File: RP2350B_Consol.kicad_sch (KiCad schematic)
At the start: 33 parts, among them J1 Conn_01x15_Socket, J10 VGA, J2 Conn_01x15_Socket, J3 Conn_01x15_Socket, J4 Conn_01x15_Socket, J5 Conn_02x06_Odd_Even, J6 Conn_02x20_Odd_Even, J7 NES_Joystick1, J8 NES_Joystick2, J9 PJ320D, U2 SN76489AN

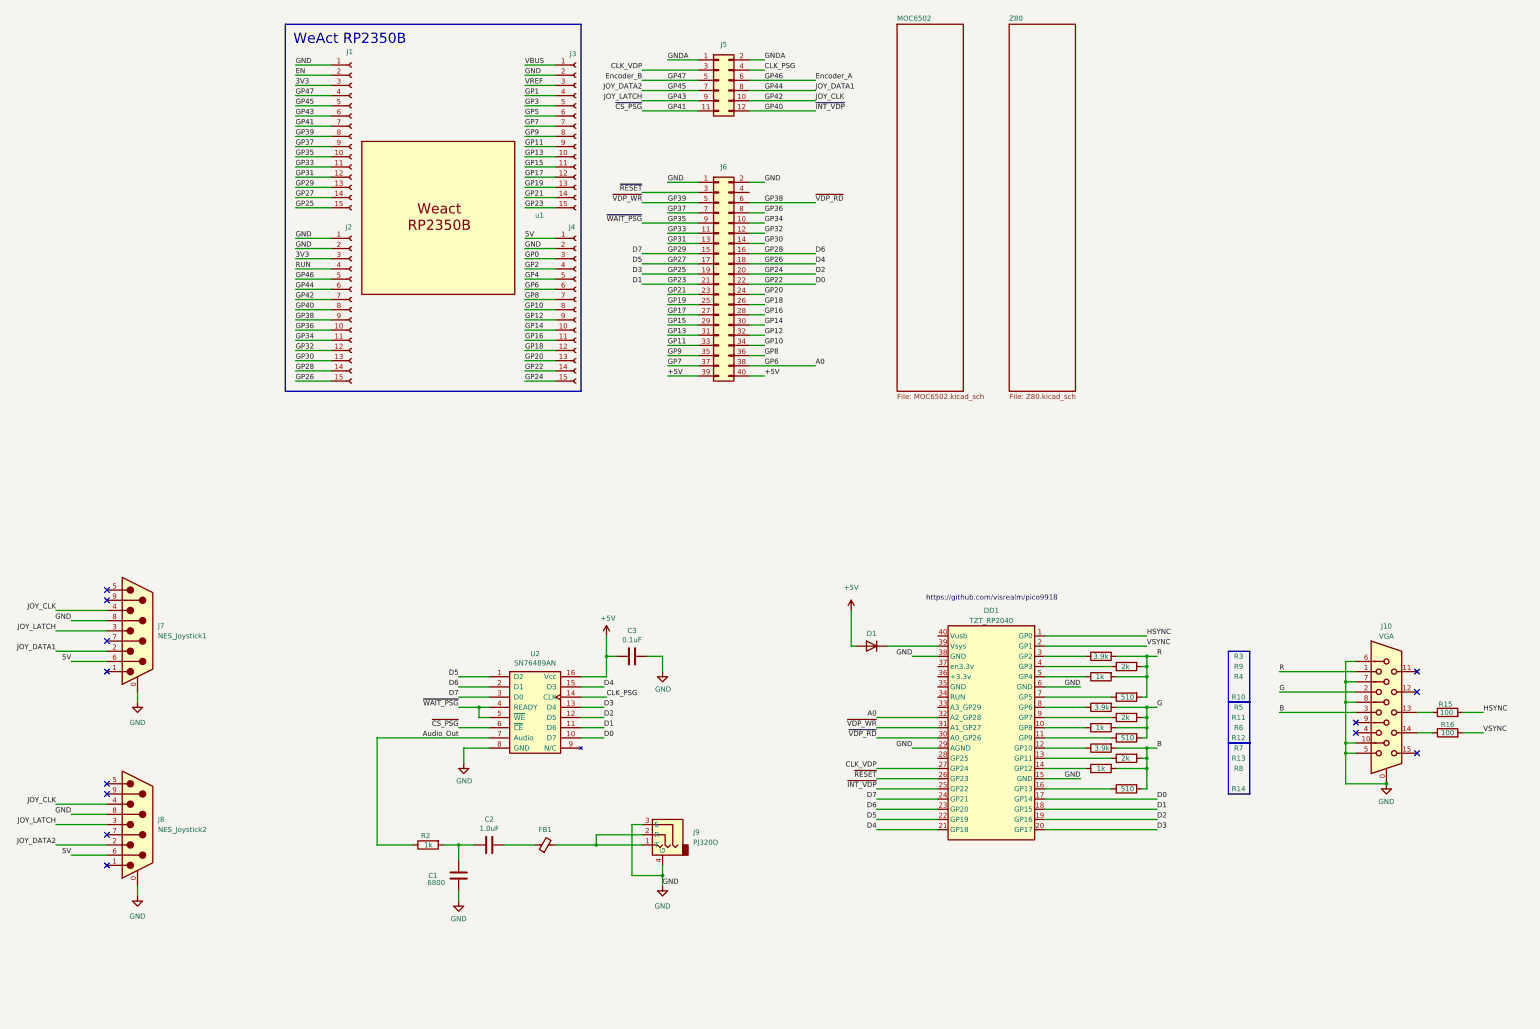
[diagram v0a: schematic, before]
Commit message: Update RP2350B_Consol.kicad_sch
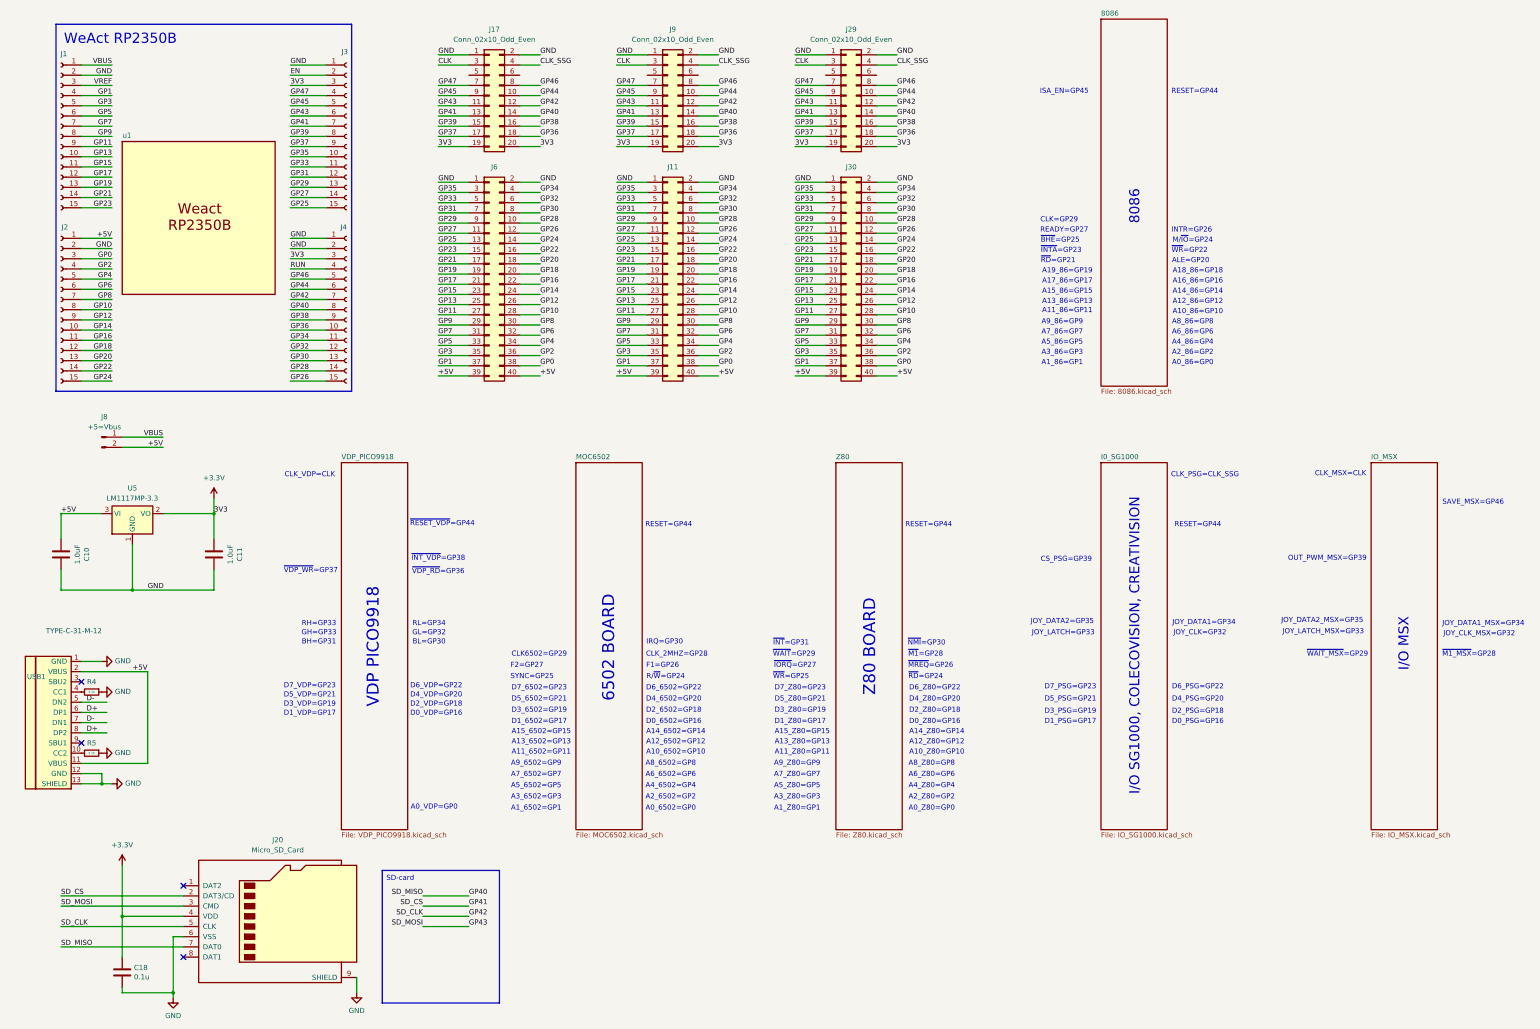
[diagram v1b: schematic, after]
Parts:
- removed C1: 6800, Capacitor_SMD:C_0805_2012Metric_Pad1.18x1.45mm_HandSolder, symbol Device:C
- removed C2: 1.0uF, Capacitor_SMD:C_0805_2012Metric_Pad1.18x1.45mm_HandSolder, symbol Device:C
- removed C3: 0.1uF, Capacitor_SMD:C_0805_2012Metric_Pad1.18x1.45mm_HandSolder, symbol Device:C
- removed D1: D, Diode_SMD:D_1206_3216Metric_Pad1.42x1.75mm_HandSolder, symbol Device:D
- removed DD1: TZT_RP2040, Library:RP2040_purple_allPin, symbol Watapico:GreatztRP2040_Purple
- removed FB1: FerriteBead_Small, Inductor_SMD:L_0805_2012Metric_Pad1.15x1.40mm_HandSolder, symbol Device:FerriteBead_Small
- removed J10: VGA, Connector_Dsub:DSUB-15-HD_Female_Horizontal_P2.29x1.98mm_EdgePinOffset3.03mm_Housed_MountingHolesOffset4.94mm, symbol Connector:DB15_Female_HighDensity_MountingHoles
- removed J5: Conn_02x06_Odd_Even, UM6502:EDGE_2x12, symbol Connector_Generic:Conn_02x06_Odd_Even
- removed J7: NES_Joystick1, Connector_Dsub:DSUB-9_Male_Vertical_P2.77x2.84mm_MountingHoles, symbol Connector:DE9_Plug_MountingHoles
- removed J8: NES_Joystick2, Connector_Dsub:DSUB-9_Male_Vertical_P2.77x2.84mm_MountingHoles, symbol Connector:DE9_Plug_MountingHoles
- removed J9: PJ320D, Library:PJ320D_3.5mm_Jack, symbol Connector_Audio:AudioJack3_Ground
- removed R10, R12, R14: 510, Resistor_SMD:R_0805_2012Metric_Pad1.20x1.40mm_HandSolder, symbol Device:R
- removed R11, R13, R9: 2k, Resistor_SMD:R_0805_2012Metric_Pad1.20x1.40mm_HandSolder, symbol Device:R
- removed R15, R16: 100, Resistor_SMD:R_0805_2012Metric_Pad1.20x1.40mm_HandSolder, symbol Device:R
- removed R2, R4, R6, R8: 1k, Resistor_SMD:R_0805_2012Metric_Pad1.20x1.40mm_HandSolder, symbol Device:R
- removed R3, R5, R7: 3.9k, Resistor_SMD:R_0805_2012Metric_Pad1.20x1.40mm_HandSolder, symbol Device:R
- removed U2: SN76489AN, Package_DIP:DIP-16_W7.62mm_LongPads, symbol LeakoChips:SN76489AN
- added C10, C11: 1.0uF, Capacitor_SMD:C_0805_2012Metric_Pad1.18x1.45mm_HandSolder, symbol Device:C
- added C18: 0.1u, Capacitor_SMD:C_0805_2012Metric_Pad1.18x1.45mm_HandSolder, symbol Device:C
- added J11, J30: Conn_02x20_Odd_Even, Connector_PinSocket_2.54mm:PinSocket_2x20_P2.54mm_Vertical, symbol Connector_Generic:Conn_02x20_Odd_Even
- added J17, J29, J9: Conn_02x10_Odd_Even, Connector_PinSocket_2.54mm:PinSocket_2x10_P2.54mm_Vertical, symbol Connector_Generic:Conn_02x10_Odd_Even
- added J20: Micro_SD_Card, Library:GCT-MEM2055-00-190-01-A, symbol Connector:Micro_SD_Card
- added J8: +5=Vbus, Connector_PinHeader_2.54mm:PinHeader_1x02_P2.54mm_Vertical, symbol Connector:Conn_01x02_Pin
- added R4, R5: 5.1K, Resistor_SMD:R_0805_2012Metric_Pad1.20x1.40mm_HandSolder, symbol Device:R_Small
- added U5: LM1117MP-3.3, Package_TO_SOT_SMD:SOT-223-3_TabPin2, symbol Regulator_Linear:LM1117MP-3.3
- added USB1: TYPE-C-31-M-12, Library:USB-TYPE-C-31-M-12_lib2, symbol Type-C:HRO-TYPE-C-31-M-12
- J6: footprint UM6502:EDGE_2x20 -> Connector_PinSocket_2.54mm:PinSocket_2x20_P2.54mm_Vertical
- u1: footprint RP2350B_WeAct:RP2350B_WeAct -> Library:RP2350B_WeAct
- renumbered J3 to J1, J4 to J2, J1 to J3, J2 to J4
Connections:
- net 5V is gone; now on net +5V: J2.1 (Pin_1)
- net ~{RESET} is gone; now on net GP35: J6.3 (Pin_3)
- net +5V: now also C10.2, J11.39 (Pin_39), J11.40 (Pin_40), J30.39 (Pin_39), J30.40 (Pin_40), J8.2 (Pin_2), U5.3 (VI), USB1.11 (VBUS), USB1.2 (VBUS)
- net GND: now also C10.1, C11.1, C18.2, J11.1 (Pin_1), J11.2 (Pin_2), J17.1 (Pin_1), J17.2 (Pin_2), J20.6 (VSS), J20.9 (SHIELD), J29.1 (Pin_1), J29.2 (Pin_2), J30.1 (Pin_1), J30.2 (Pin_2), J9.1 (Pin_1), J9.2 (Pin_2), R4.1, R5.1, U5.1 (GND), USB1.1 (GND), USB1.12 (GND), USB1.13 (SHIELD)
- net GP0: now also J6.38 (Pin_38), J11.38 (Pin_38), J30.38 (Pin_38)
- net GP1: now also J6.37 (Pin_37), J11.37 (Pin_37), J30.37 (Pin_37)
- net GP10: now also J6.28 (Pin_28), J11.28 (Pin_28), J30.28 (Pin_28); no longer J6.34 (Pin_34)
- net GP11: now also J6.27 (Pin_27), J11.27 (Pin_27), J30.27 (Pin_27); no longer J6.33 (Pin_33)
- net GP12: now also J6.26 (Pin_26), J11.26 (Pin_26), J30.26 (Pin_26); no longer J6.32 (Pin_32)
- net GP13: now also J6.25 (Pin_25), J11.25 (Pin_25), J30.25 (Pin_25); no longer J6.31 (Pin_31)
- net GP14: now also J6.24 (Pin_24), J11.24 (Pin_24), J30.24 (Pin_24); no longer J6.30 (Pin_30)
- net GP15: now also J6.23 (Pin_23), J11.23 (Pin_23), J30.23 (Pin_23); no longer J6.29 (Pin_29)
- net GP16: now also J6.22 (Pin_22), J11.22 (Pin_22), J30.22 (Pin_22); no longer J6.28 (Pin_28)
- net GP17: now also J6.21 (Pin_21), J11.21 (Pin_21), J30.21 (Pin_21); no longer J6.27 (Pin_27)
- net GP18: now also J6.20 (Pin_20), J11.20 (Pin_20), J30.20 (Pin_20); no longer J6.26 (Pin_26)
- net GP19: now also J6.19 (Pin_19), J11.19 (Pin_19), J30.19 (Pin_19); no longer J6.25 (Pin_25)
- net GP2: now also J6.36 (Pin_36), J11.36 (Pin_36), J30.36 (Pin_36)
- net GP20: now also J6.18 (Pin_18), J11.18 (Pin_18), J30.18 (Pin_18); no longer J6.24 (Pin_24)
- net GP21: now also J6.17 (Pin_17), J11.17 (Pin_17), J30.17 (Pin_17); no longer J6.23 (Pin_23)
- net GP3: now also J6.35 (Pin_35), J11.35 (Pin_35), J30.35 (Pin_35)
- net GP30: now also J6.8 (Pin_8), J11.8 (Pin_8), J30.8 (Pin_8); no longer J6.14 (Pin_14)
- net GP31: now also J6.7 (Pin_7), J11.7 (Pin_7), J30.7 (Pin_7); no longer J6.13 (Pin_13)
- net GP32: now also J6.6 (Pin_6), J11.6 (Pin_6), J30.6 (Pin_6); no longer J6.12 (Pin_12)
- net GP33: now also J6.5 (Pin_5), J11.5 (Pin_5), J30.5 (Pin_5); no longer J6.11 (Pin_11)
- net GP34: now also J6.4 (Pin_4), J11.4 (Pin_4), J30.4 (Pin_4); no longer J6.10 (Pin_10)
- net GP35: now also J11.3 (Pin_3), J30.3 (Pin_3); no longer J6.9 (Pin_9)
- net GP36: now also J17.18 (Pin_18), J29.18 (Pin_18), J9.18 (Pin_18); no longer J6.8 (Pin_8)
- net GP37: now also J17.17 (Pin_17), J29.17 (Pin_17), J9.17 (Pin_17); no longer J6.7 (Pin_7)
- net GP38: now also J17.16 (Pin_16), J29.16 (Pin_16), J9.16 (Pin_16); no longer J6.6 (Pin_6)
- net GP39: now also J17.15 (Pin_15), J29.15 (Pin_15), J9.15 (Pin_15); no longer J6.5 (Pin_5)
- net GP4: now also J6.34 (Pin_34), J11.34 (Pin_34), J30.34 (Pin_34)
- net GP40: now also J17.14 (Pin_14), J20.7 (DAT0), J29.14 (Pin_14), J9.14 (Pin_14)
- net GP41: now also J17.13 (Pin_13), J20.2 (DAT3/CD), J29.13 (Pin_13), J9.13 (Pin_13)
- net GP42: now also J17.12 (Pin_12), J20.5 (CLK), J29.12 (Pin_12), J9.12 (Pin_12)
- net GP43: now also J17.11 (Pin_11), J20.3 (CMD), J29.11 (Pin_11), J9.11 (Pin_11)
- net GP44: now also J17.10 (Pin_10), J29.10 (Pin_10), J9.10 (Pin_10)
- net GP45: now also J17.9 (Pin_9), J29.9 (Pin_9), J9.9 (Pin_9)
- net GP5: now also J6.33 (Pin_33), J11.33 (Pin_33), J30.33 (Pin_33)
- net GP7: now also J6.31 (Pin_31), J11.31 (Pin_31), J30.31 (Pin_31); no longer J6.37 (Pin_37)
- net GP8: now also J6.30 (Pin_30), J11.30 (Pin_30), J30.30 (Pin_30); no longer J6.36 (Pin_36)
- net GP9: now also J6.29 (Pin_29), J11.29 (Pin_29), J30.29 (Pin_29); no longer J6.35 (Pin_35)
- net VBUS: now also J8.1 (Pin_1)
- net 3V3 renamed +3.3V
- net +3.3V: now also C11.2, C18.1, J17.19 (Pin_19), J17.20 (Pin_20), J20.4 (VDD), J29.19 (Pin_19), J29.20 (Pin_20), J9.19 (Pin_19), J9.20 (Pin_20), U5.2 (VO)
- net A0 renamed GP6
- net GP6: now also J6.32 (Pin_32), J11.32 (Pin_32), J30.32 (Pin_32); no longer J6.38 (Pin_38)
- net D0 renamed GP22
- net GP22: now also J6.16 (Pin_16), J11.16 (Pin_16), J30.16 (Pin_16); no longer J6.22 (Pin_22)
- net D1 renamed GP23
- net GP23: now also J6.15 (Pin_15), J11.15 (Pin_15), J30.15 (Pin_15); no longer J6.21 (Pin_21)
- net D2 renamed GP24
- net GP24: now also J6.14 (Pin_14), J11.14 (Pin_14), J30.14 (Pin_14); no longer J6.20 (Pin_20)
- net D3 renamed GP25
- net GP25: now also J6.13 (Pin_13), J11.13 (Pin_13), J30.13 (Pin_13); no longer J6.19 (Pin_19)
- net D4 renamed GP26
- net GP26: now also J6.12 (Pin_12), J11.12 (Pin_12), J30.12 (Pin_12); no longer J6.18 (Pin_18)
- net D5 renamed GP27
- net GP27: now also J6.11 (Pin_11), J11.11 (Pin_11), J30.11 (Pin_11); no longer J6.17 (Pin_17)
- net D6 renamed GP28
- net GP28: now also J6.10 (Pin_10), J11.10 (Pin_10), J30.10 (Pin_10); no longer J6.16 (Pin_16)
- net D7 renamed GP29
- net GP29: now also J6.9 (Pin_9), J11.9 (Pin_9), J30.9 (Pin_9); no longer J6.15 (Pin_15)
- net Encoder_A renamed GP46
- net GP46: now also J17.8 (Pin_8), J29.8 (Pin_8), J9.8 (Pin_8)
- net Encoder_B renamed GP47
- net GP47: now also J17.7 (Pin_7), J29.7 (Pin_7), J9.7 (Pin_7)
- new net: R4.2, USB1.4 (CC1)
- new net: R5.2, USB1.10 (CC2)
- new net CLK: J17.3 (Pin_3), J29.3 (Pin_3), J9.3 (Pin_3)
- new net CLK_SSG: J17.4 (Pin_4), J29.4 (Pin_4), J9.4 (Pin_4)
- new net D+: USB1.6 (DP1), USB1.8 (DP2)
- new net D-: USB1.5 (DN2), USB1.7 (DN1)
- no-connect marks 13 -> 4
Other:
- added sheet 8086 (8086.kicad_sch)
- added sheet I0_SG1000 (IO_SG1000.kicad_sch)
- added sheet IO_MSX (IO_MSX.kicad_sch)
- added sheet VDP_PICO9918 (VDP_PICO9918.kicad_sch)
- note added: "6502 BOARD"
- note added: "8086"
- note added: "A0_6502=GP0"
- note added: "A0_86=GP0"
- note added: "A0_VDP=GP0"
- note added: "A0_Z80=GP0"
- note added: "A10_6502=GP10"
- note added: "A10_86=GP10"
- note added: "A10_Z80=GP10"
- note added: "A11_6502=GP11"
- note added: "A11_86=GP11"
- note added: "A11_Z80=GP11"
- note added: "A12_6502=GP12"
- note added: "A12_86=GP12"
- note added: "A12_Z80=GP12"
- note added: "A13_6502=GP13"
- note added: "A13_86=GP13"
- note added: "A13_Z80=GP13"
- note added: "A14_6502=GP14"
- note added: "A14_86=GP14"
- note added: "A14_Z80=GP14"
- note added: "A15_6502=GP15"
- note added: "A15_86=GP15"
- note added: "A15_Z80=GP15"
- note added: "A16_86=GP16"
- note added: "A17_86=GP17"
- note added: "A18_86=GP18"
- note added: "A19_86=GP19"
- note added: "A1_6502=GP1"
- note added: "A1_86=GP1"
- note added: "A1_Z80=GP1"
- note added: "A2_6502=GP2"
- note added: "A2_86=GP2"
- note added: "A2_Z80=GP2"
- note added: "A3_6502=GP3"
- note added: "A3_86=GP3"
- note added: "A3_Z80=GP3"
- note added: "A4_6502=GP4"
- note added: "A4_86=GP4"
- note added: "A4_Z80=GP4"
- note added: "A5_6502=GP5"
- note added: "A5_86=GP5"
- note added: "A5_Z80=GP5"
- note added: "A6_6502=GP6"
- note added: "A6_86=GP6"
- note added: "A6_Z80=GP6"
- note added: "A7_6502=GP7"
- note added: "A7_86=GP7"
- note added: "A7_Z80=GP7"
- note added: "A8_6502=GP8"
- note added: "A8_86=GP8"
- note added: "A8_Z80=GP8"
- note added: "A9_6502=GP9"
- note added: "A9_86=GP9"
- note added: "A9_Z80=GP9"
- note added: "ALE=GP20"
- note added: "BH=GP31"
- note added: "BL=GP30"
- note added: "CLK6502=GP29"
- note added: "CLK=GP29"
- note added: "CLK_2MHZ=GP28"
- note added: "CLK_MSX=CLK"
- note added: "CLK_PSG=CLK_SSG"
- note added: "CLK_VDP=CLK"
- note added: "CS_PSG=GP39"
- note added: "D0_6502=GP16"
- note added: "D0_PSG=GP16"
- note added: "D0_VDP=GP16"
- note added: "D0_Z80=GP16"
- note added: "D1_6502=GP17"
- note added: "D1_PSG=GP17"
- note added: "D1_VDP=GP17"
- note added: "D1_Z80=GP17"
- note added: "D2_6502=GP18"
- note added: "D2_PSG=GP18"
- note added: "D2_VDP=GP18"
- note added: "D2_Z80=GP18"
- note added: "D3_6502=GP19"
- note added: "D3_PSG=GP19"
- note added: "D3_VDP=GP19"
- note added: "D3_Z80=GP19"
- note added: "D4_6502=GP20"
- note added: "D4_PSG=GP20"
- note added: "D4_VDP=GP20"
- note added: "D4_Z80=GP20"
- note added: "D5_6502=GP21"
- note added: "D5_PSG=GP21"
- note added: "D5_VDP=GP21"
- note added: "D5_Z80=GP21"
- note added: "D6_6502=GP22"
- note added: "D6_PSG=GP22"
- note added: "D6_VDP=GP22"
- note added: "D6_Z80=GP22"
- note added: "D7_6502=GP23"
- note added: "D7_PSG=GP23"
- note added: "D7_VDP=GP23"
- note added: "D7_Z80=GP23"
- note added: "F1=GP26"
- note added: "F2=GP27"
- note added: "GH=GP33"
- note added: "GL=GP32"
- note added: "I/O MSX"
- note added: "I/O SG1000, COLECOVISION, CREATIVISION"
- note added: "INTR=GP26"
- note added: "IRQ=GP30"
- note added: "ISA_EN=GP45"
- note added: "JOY_CLK=GP32"
- note added: "JOY_CLK_MSX=GP32"
- note added: "JOY_DATA1=GP34"
- note added: "JOY_DATA1_MSX=GP34"
- note added: "JOY_DATA2=GP35"
- note added: "JOY_DATA2_MSX=GP35"
- note added: "JOY_LATCH=GP33"
- note added: "JOY_LATCH_MSX=GP33"
- note added: "M/~{IO}=GP24"
- note added: "OUT_PWM_MSX=GP39"
- note added: "R/~{W}=GP24"
- note added: "READY=GP27"
- note added: "RESET=GP44"
- note added: "RH=GP33"
- note added: "RL=GP34"
- note added: "SAVE_MSX=GP46"
- note added: "SYNC=GP25"
- note added: "VDP PICO9918"
- note added: "Z80 BOARD"
- note added: "~{BHE}=GP25"
- note added: "~{INTA}=GP23"
- note added: "~{INT_VDP}=GP38"
- note added: "~{INT}=GP31"
- note added: "~{IORQ}=GP27"
- note added: "~{M1_MSX}=GP28"
- note added: "~{M1}=GP28"
- note added: "~{MREQ}=GP26"
- note added: "~{NMI}=GP30"
- note added: "~{RD}=GP21"
- note added: "~{RD}=GP24"
- note added: "~{RESET_VDP}=GP44"
- note added: "~{VDP_RD}=GP36"
- note added: "~{VDP_WR}=GP37"
- note added: "~{WAIT_MSX}=GP29"
- note added: "~{WAIT}=GP29"
- note added: "~{WR}=GP22"
- note added: "~{WR}=GP25"
- note removed: "https://github.com/visrealm/pico9918"
- moved on the sheet: J1, J2, J3, J4, J6, u1
